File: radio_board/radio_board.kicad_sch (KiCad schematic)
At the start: 86 parts, among them CN1 HX JN1.27-2X5P ZZ H4.9, Q1 2N7002K, SW2 RKB2SJG250SMTRLFS, SW3 MSK12C02, U1 FSC-BT1036C, U2 TP4057, U3 XB5352A, U4 SKB369, U5 S2B-PH-K-S(LF)(SN), U6 XC6206P332MR

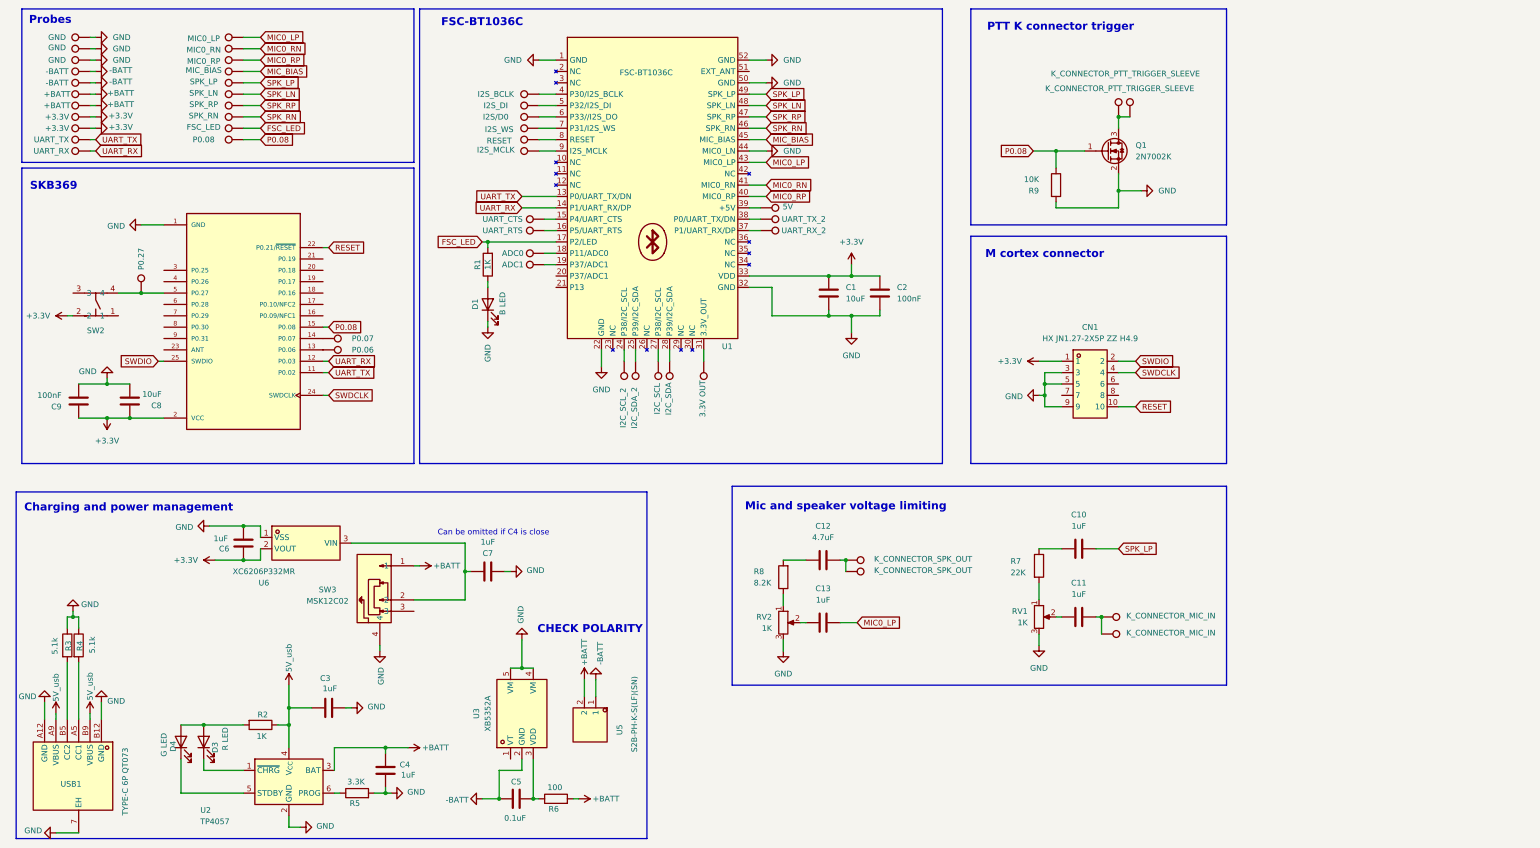
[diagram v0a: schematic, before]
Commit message: [Feature] WIP radio board
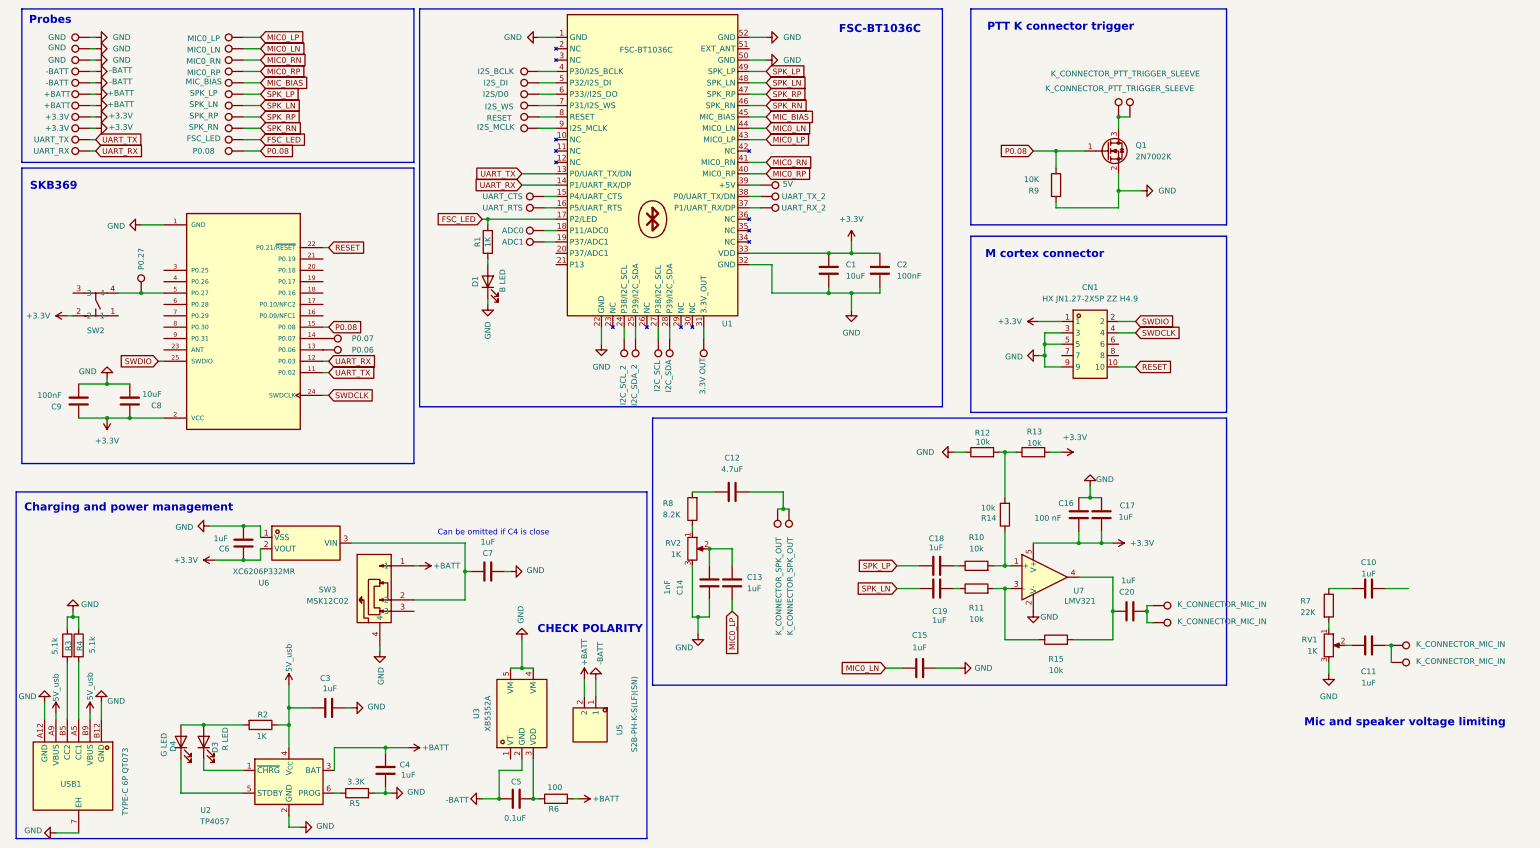
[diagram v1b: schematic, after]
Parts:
- added C14: 1nF, Capacitor_SMD:C_0603_1608Metric_Pad1.08x0.95mm_HandSolder, symbol Device:C
- added C15: 1uF, Capacitor_SMD:C_0603_1608Metric_Pad1.08x0.95mm_HandSolder, symbol Device:C
- added C16: 100 nF, Resistor_SMD:R_0603_1608Metric_Pad0.98x0.95mm_HandSolder, symbol Device:C
- added C17, C18, C19, C20: 1uF, Resistor_SMD:R_0603_1608Metric_Pad0.98x0.95mm_HandSolder, symbol Device:C
- added R10, R11, R12, R13, R14, R15: 10k, Resistor_SMD:R_0603_1608Metric_Pad0.98x0.95mm_HandSolder, symbol Device:R
- added TP49: MIC0_LN, TestPoint:TestPoint_THTPad_D2.0mm_Drill1.0mm, symbol Connector:TestPoint
- added TP50: K_CONNECTOR_MIC_IN, TestPoint:TestPoint_THTPad_D2.0mm_Drill1.0mm, symbol Connector:TestPoint
- added TP51: K_CONNECTOR_MIC_IN, TestPoint:TestPoint_Pad_D3.0mm, symbol Connector:TestPoint
- added U7: LMV321, Package_TO_SOT_SMD:SOT-23-5_HandSoldering, symbol Amplifier_Operational:LMV321
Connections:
- net +3.3V: now also C16.2, C17.2, R13.2, U7.5 (V+)
- net GND: now also C14.1, C15.1, C16.1, C17.1, R12.1, U7.2 (V-); no longer U1.44 (MIC0_LN)
- net MIC0_LP: now also C13.2; no longer C13.1
- net SPK_LN: now also C19.2
- net SPK_LP: now also C18.2; no longer C10.1
- net at RV2.2: now also C13.1, C14.2; no longer C13.2
- new net: C18.1, R10.1
- new net: R10.2, R14.1, U7.1 (+)
- new net: R11.2, R15.1, U7.3 (-)
- new net: C20.1, R15.2, U7.4
- new net: C20.2, TP50.1, TP51.1
- new net: R12.2, R13.1, R14.2
- new net: C19.1, R11.1
- new net MIC0_LN: C15.2, TP49.1, U1.44 (MIC0_LN)
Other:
- moved on the sheet: C1, C10, C11, C12, C13, C2, CN1, D1, R1, R7, R8, RV1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
